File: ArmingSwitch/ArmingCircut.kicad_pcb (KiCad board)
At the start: 2 copper layers, 35.6 x 19 mm, 7 parts, among them J1 Screw_Terminal_01x02, J2 Screw_Terminal_01x02, J3 Screw_Terminal_01x02

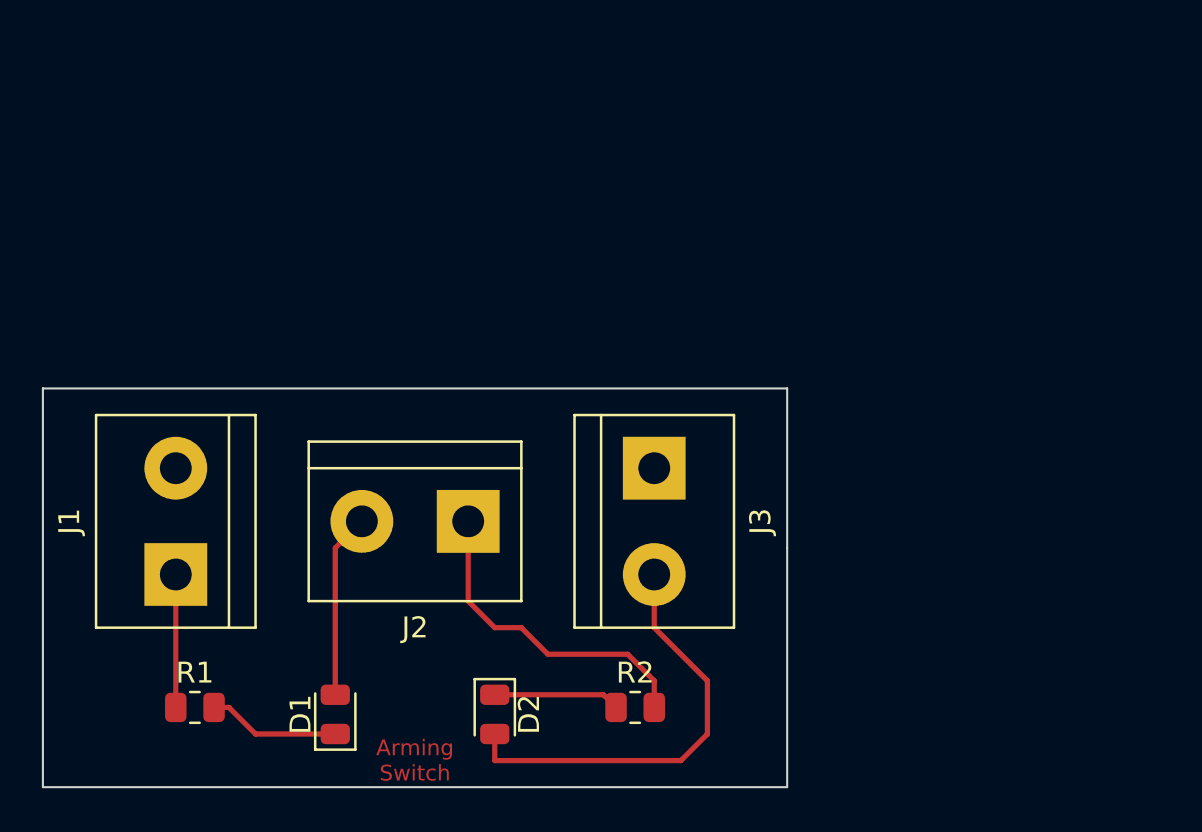
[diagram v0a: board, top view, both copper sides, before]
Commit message: no more errors!
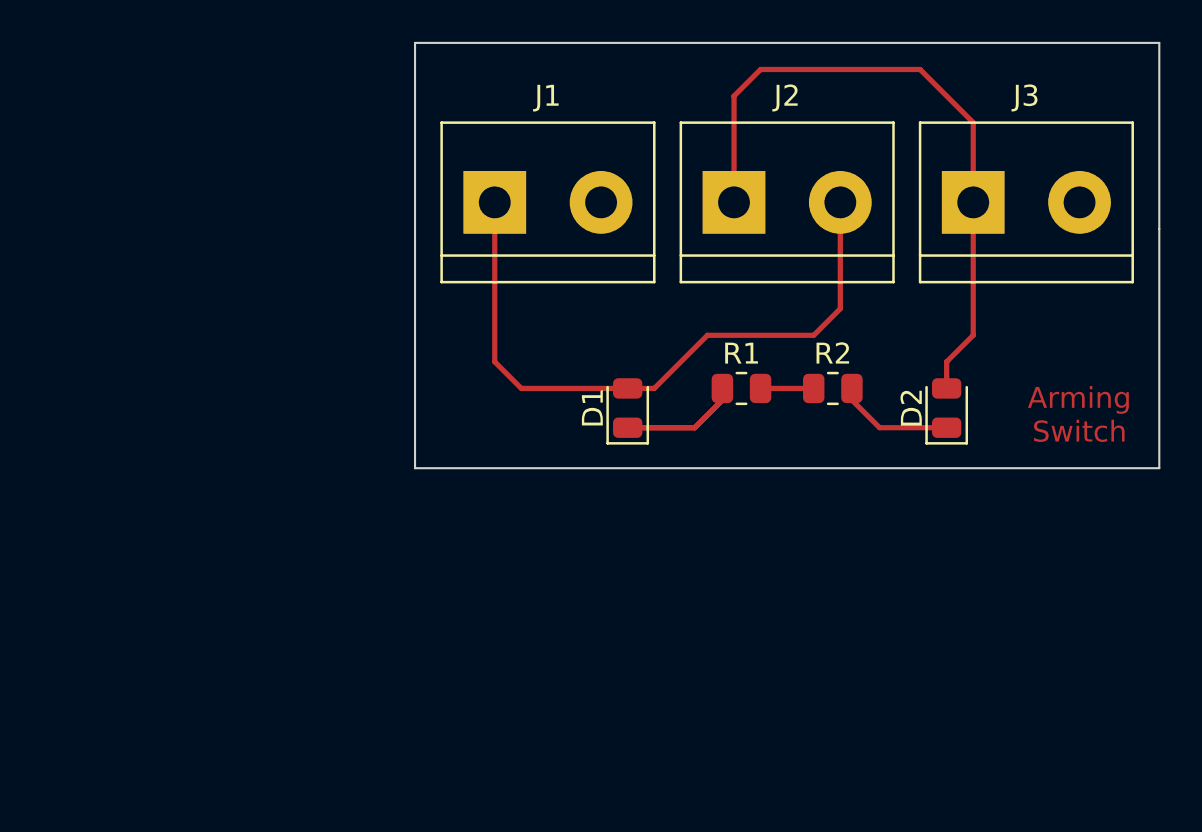
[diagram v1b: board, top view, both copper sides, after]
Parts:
- moved R1 30.2 mm to (157.8, 105.4)
- moved D2 26.1 mm to (167.6, 106.3), turned to 90 degrees
- moved J1 23.4 mm to (146.1, 96.5), turned to 0 degrees
- moved D1 20.2 mm to (152.4, 106.3)
- moved J3 19.8 mm to (168.9, 96.5), turned to 0 degrees
- moved J2 19.8 mm to (157.5, 96.5), turned to 0 degrees
- moved R2 17.9 mm to (162.2, 105.4)
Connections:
- D1 pad 1: (no net) -> Net-(D1-Pad1)
- D1 pad 2: (no net) -> Net-(D1-Pad2)
- D2 pad 1: (no net) -> Net-(D2-Pad1)
- D2 pad 2: (no net) -> Net-(D2-Pad2)
- J1 pad 1: (no net) -> Net-(D1-Pad2)
- J1 pad 2: (no net) -> +5V
- J2 pad 1: (no net) -> Net-(D2-Pad2)
- J2 pad 2: (no net) -> Net-(D1-Pad2)
- J3 pad 1: (no net) -> Net-(D2-Pad2)
- J3 pad 2: (no net) -> /ArmingSwitch/ArmingSwitch
- R1 pad 1: (no net) -> Net-(D1-Pad1)
- R1 pad 2: (no net) -> GND
- R2 pad 1: (no net) -> GND
- R2 pad 2: (no net) -> Net-(D2-Pad1)
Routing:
- net (no net): track 63.7 -> 0.00 mm
- net Net-(D2-Pad2): track 0.00 -> 31.3 mm
- net Net-(D1-Pad2): track 0.00 -> 31.3 mm
- net Net-(D1-Pad1): track 0.00 -> 11.3 mm
- net Net-(D2-Pad1): track 0.00 -> 5.63 mm
- net GND: track 0.00 -> 2.54 mm
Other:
- board size 35.6 x 19 mm -> 35.6 x 20.3 mm
